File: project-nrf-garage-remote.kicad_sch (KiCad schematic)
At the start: 4 parts, among them J1 Screw_Terminal_01x02, J2 Screw_Terminal_01x04, Q1 BSS138W, Q2 BSS138W

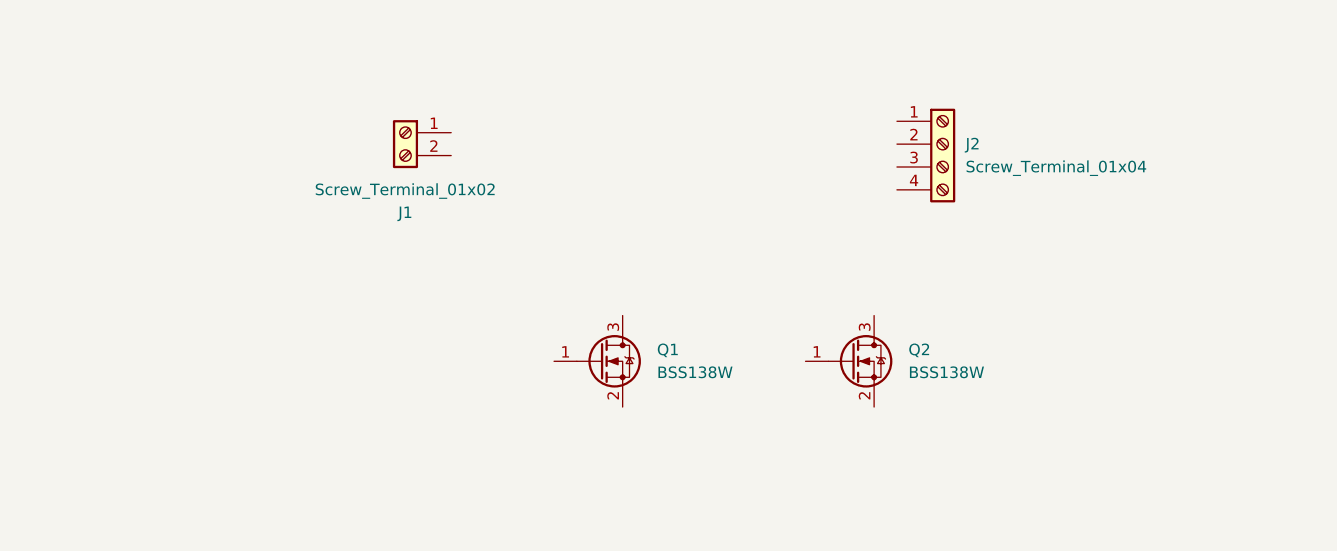
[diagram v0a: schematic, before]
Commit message: Connect schematic
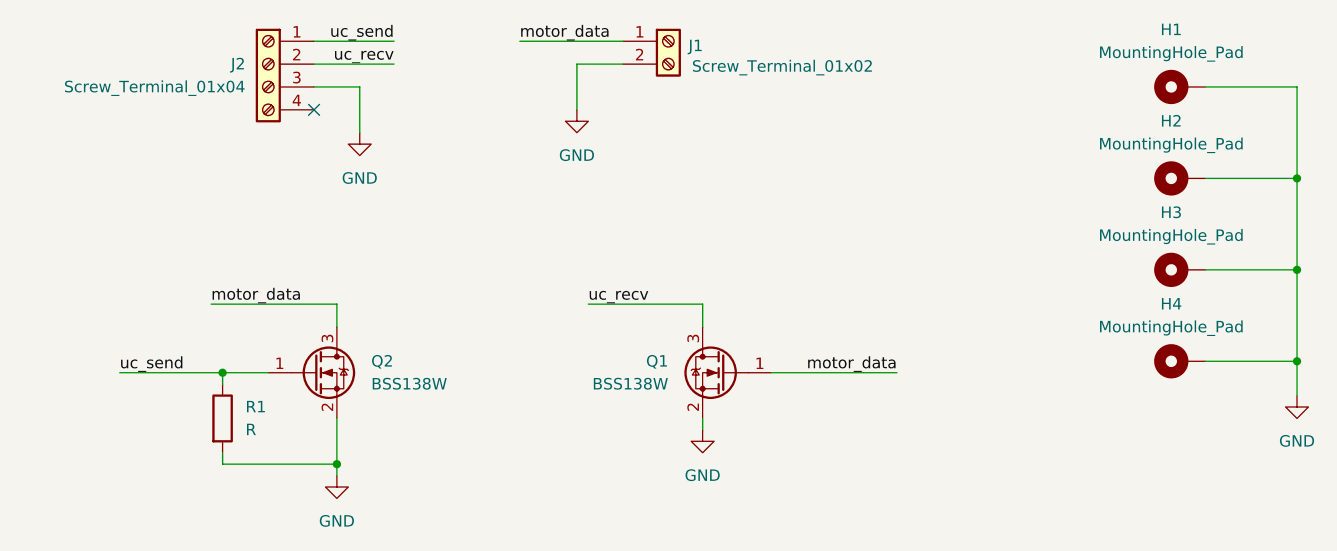
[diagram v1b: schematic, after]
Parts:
- added H1, H2, H3, H4: MountingHole_Pad, symbol Mechanical:MountingHole_Pad
- added R1: R, Resistor_SMD:R_0603_1608Metric, symbol Device:R
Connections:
- net uc_send: now reaches Q2.1 (G)
- net uc_send: now also J2.1 (Pin_1), R1.1
- net GND: now reaches Q2.2 (S)
- net GND: now also J1.2 (Pin_2), J2.3 (Pin_3), Q1.2 (S), H1.1, H2.1, H3.1, H4.1, R1.2
- net motor_data: now reaches Q2.3 (D)
- net motor_data: now also J1.1 (Pin_1), Q1.1 (G)
- net uc_recv: now reaches J2.2 (Pin_2)
- net uc_recv: now also Q1.3 (D)
- no-connect marks 0 -> 1
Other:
- moved on the sheet: J1, J2, Q1, Q2
